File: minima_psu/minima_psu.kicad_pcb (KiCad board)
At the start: 2 copper layers, 78 x 90 mm, 26 parts, among them J1 Screw_Terminal_01x03, J2 Screw_Terminal_01x02, J3 Screw_Terminal_01x03, J4 Screw_Terminal_01x03, J5 Screw_Terminal_01x03, J6 Screw_Terminal_01x03

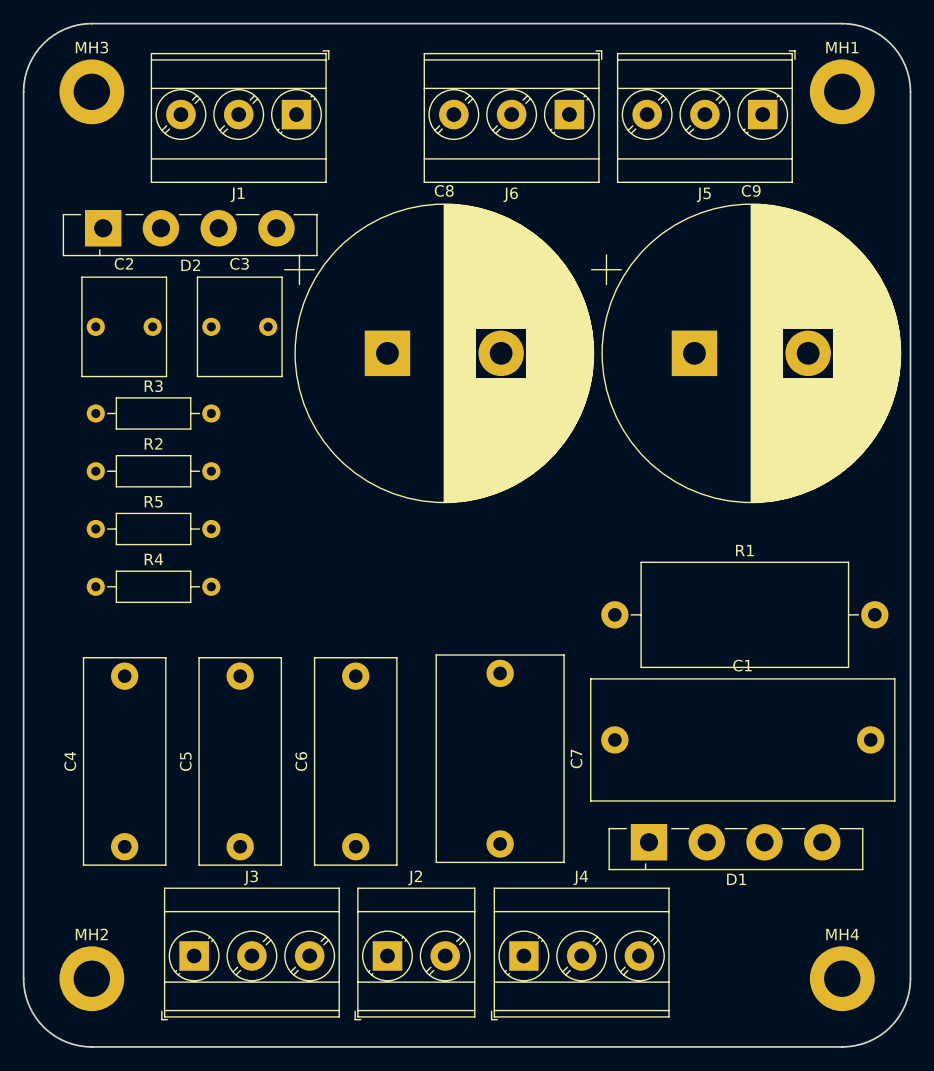
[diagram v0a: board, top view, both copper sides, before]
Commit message: Minor PCB adjustements
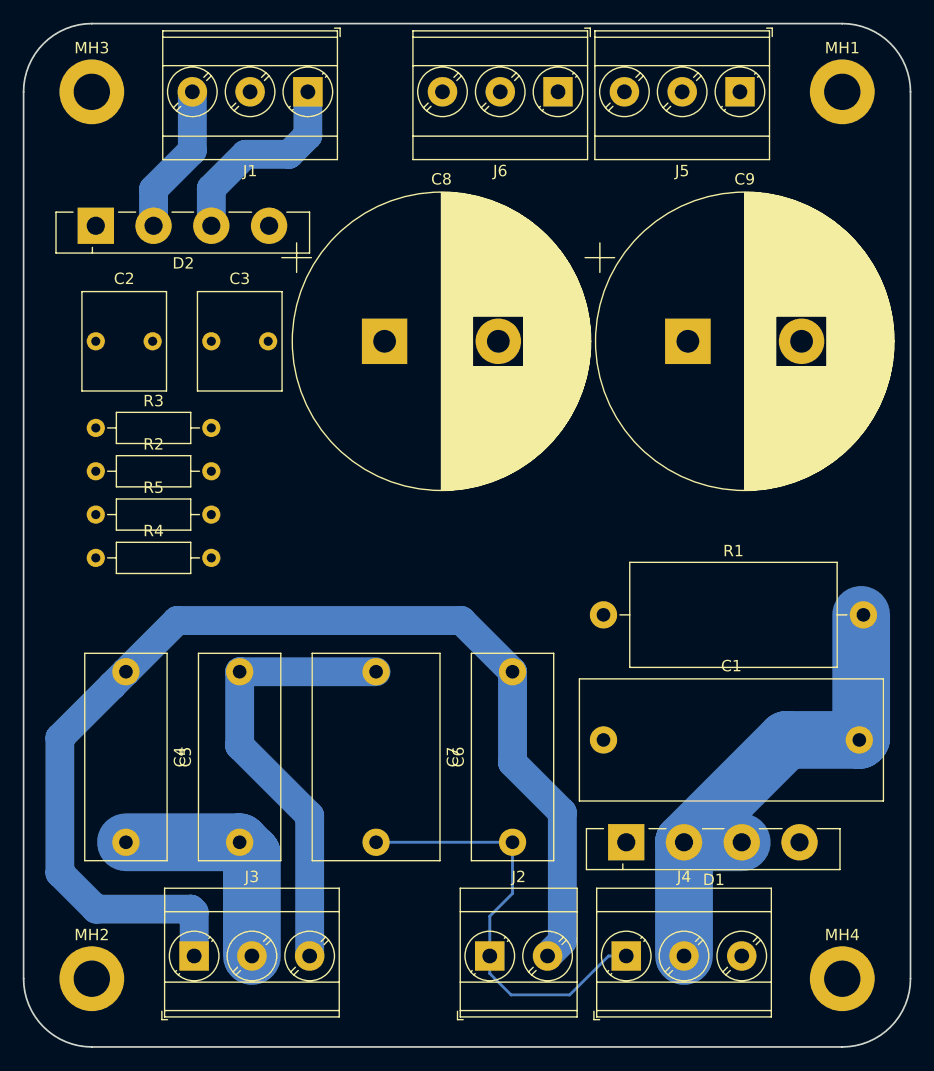
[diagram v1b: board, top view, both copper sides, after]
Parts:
- moved C4 15.4 mm to (104.2, 126.8), turned to 270 degrees
- moved C6 13.8 mm to (138.2, 141.8)
- moved C7 10.9 mm to (126.2, 126.8)
- moved J2 9.00 mm to (136.2, 151.8)
- moved J4 9.00 mm to (148.2, 151.8)
- moved J5 2.83 mm to (158.2, 75.8)
- moved R4 2.54 mm to (101.6, 116.8)
- moved J1 2.24 mm to (120.2, 75.8)
- moved J6 2.24 mm to (142.2, 75.8)
- moved D1 2.00 mm to (148.2, 141.8)
- moved C2 1.27 mm to (101.6, 97.8)
- moved C3 1.27 mm to (111.8, 97.8)
- moved R3 1.27 mm to (101.6, 105.4)
- moved R5 1.27 mm to (101.6, 113.0)
- moved C9 1.21 mm to (153.7, 97.8)
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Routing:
- net /ac_l: track 0.00 -> 102.3 mm
- net Earth_Protective: track 0.00 -> 65.7 mm
- net /ac_n: track 0.00 -> 39.6 mm
- net Net-(C6-Pad1): track 0.00 -> 38.6 mm
- net Net-(C2-Pad1): track 0.00 -> 17.5 mm
- net Net-(C3-Pad2): track 0.00 -> 13.2 mm
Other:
- net class ac_p added: clearance 2, trace_width 2.54, via_dia 0.8, via_drill 0.4
- net class ac_prot added: clearance 2, trace_width 5.08, via_dia 0.8, via_drill 0.4
- net class dc_p added: clearance 1, trace_width 5.08, via_dia 0.8, via_drill 0.4
